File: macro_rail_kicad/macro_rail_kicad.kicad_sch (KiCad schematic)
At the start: 15 parts, among them J1 Battery, J2 Motor, J3 128x128 OLED, J4 GIMBAL, SW1 POWER, SW2 SHUTTER, SW3 PREVIOUS, SW4 NEXT, SW5 RESET, U1 Pico, U2 LM7805

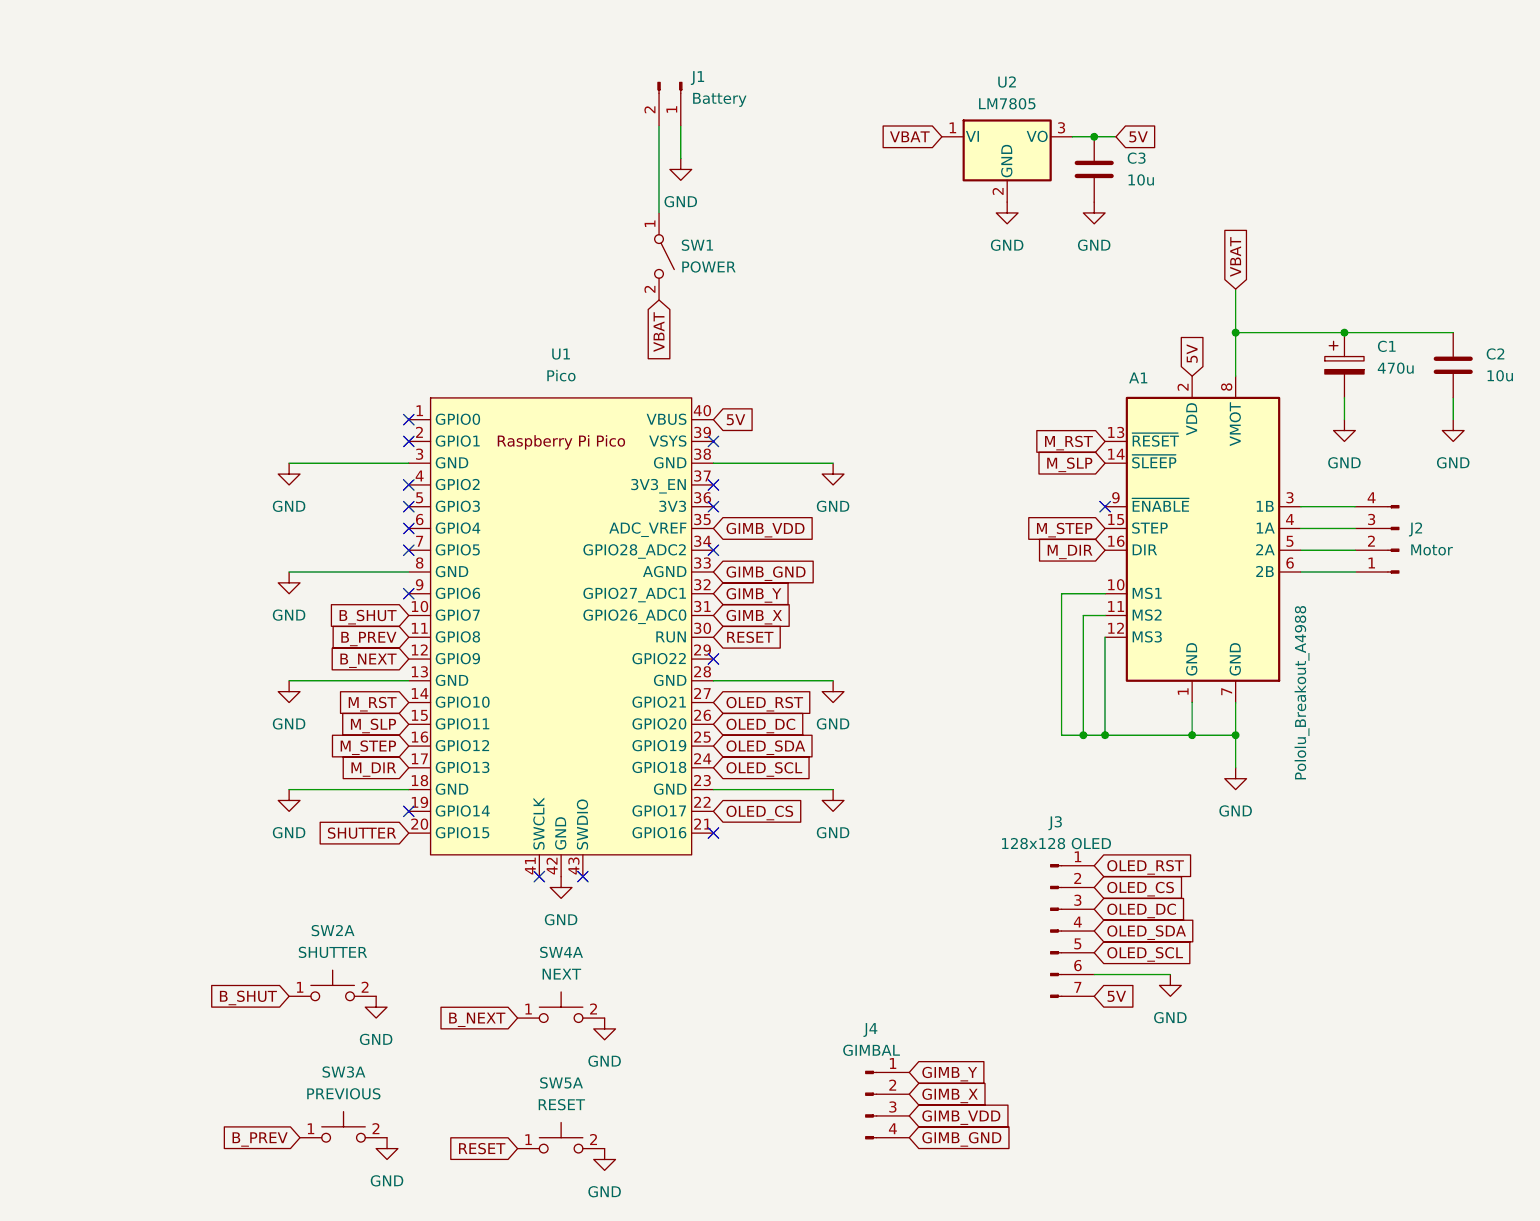
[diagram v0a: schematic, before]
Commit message: Organized schematic.
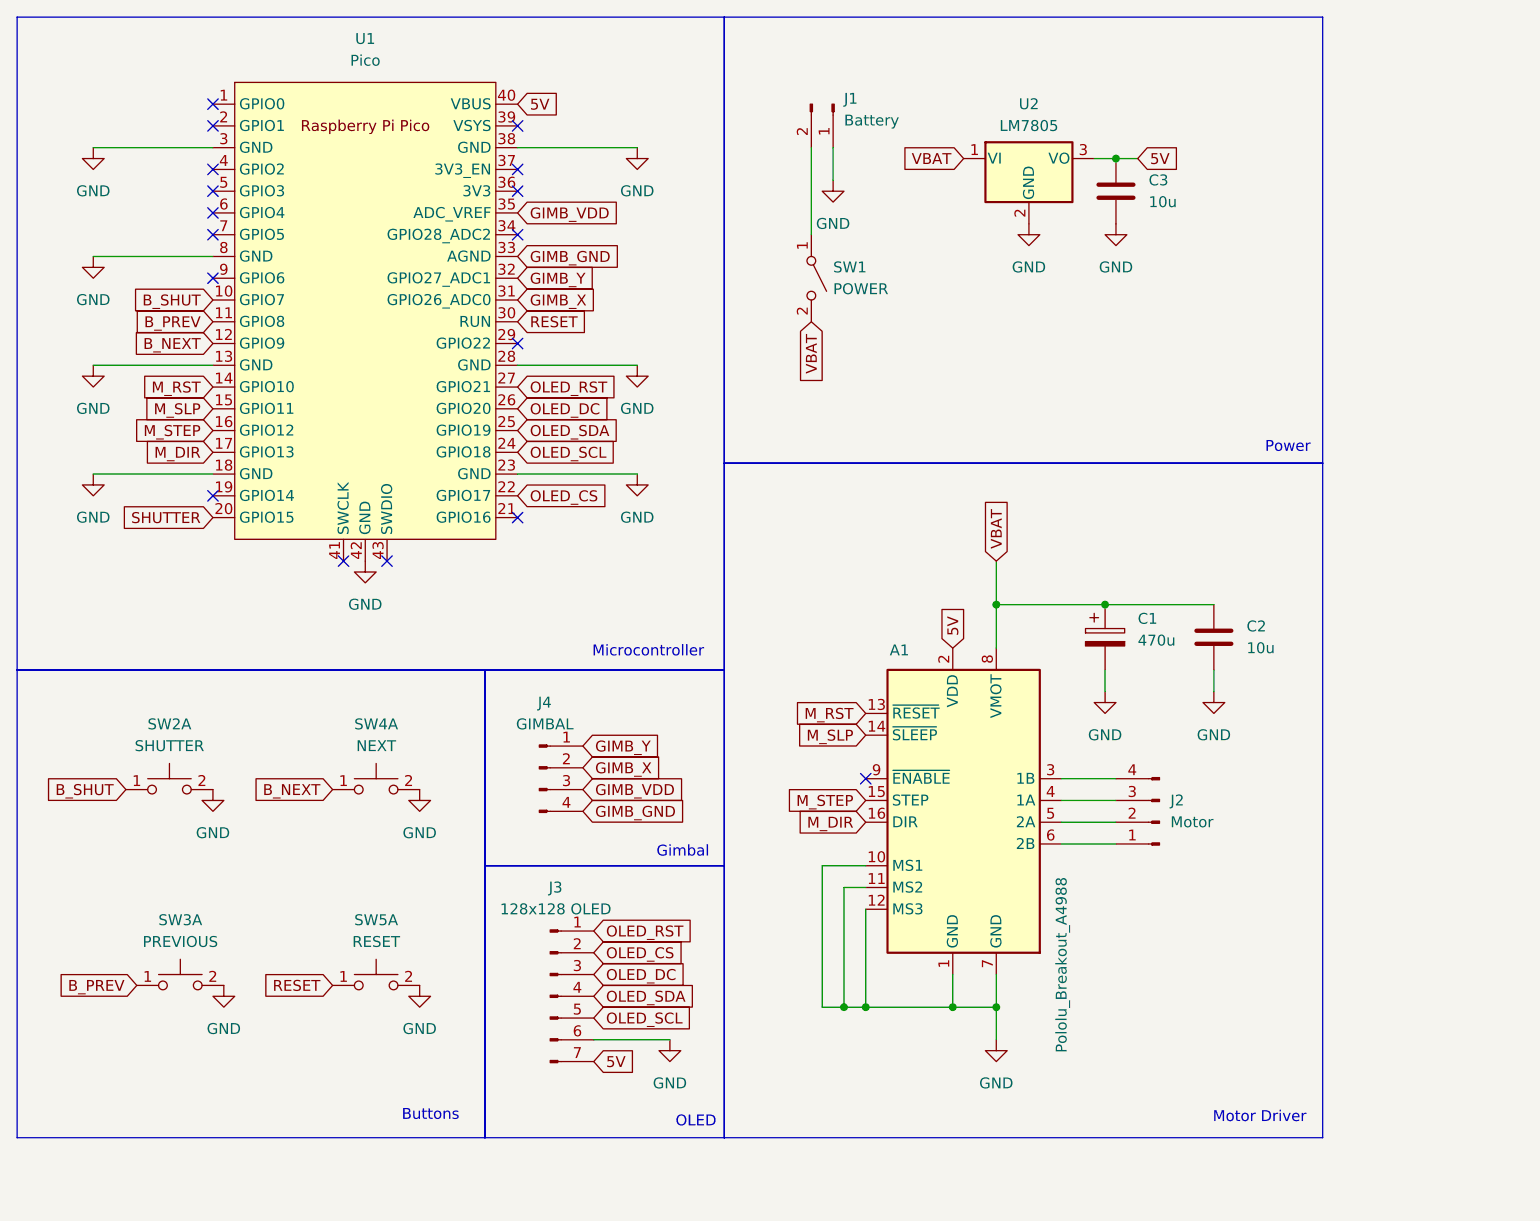
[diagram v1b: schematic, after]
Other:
- note added: "Buttons"
- note added: "Gimbal"
- note added: "Microcontroller"
- note added: "Motor Driver"
- note added: "OLED"
- note added: "Power"
- moved on the sheet: A1, C1, C2, C3, J1, J2, J3, J4, SW1, SW2A, SW3A, SW4A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
